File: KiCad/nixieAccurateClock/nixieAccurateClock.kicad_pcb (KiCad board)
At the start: 2 copper layers, 153 x 101.5 mm, 23 parts, among them J1 Conn_01x02_Pin, J2 Conn_01x02_Pin, J3 Conn_01x02_Pin, J4 Conn_Coaxial, Q1 PZTA42, SW1 SW_DIP_x02, U2 PX1125T

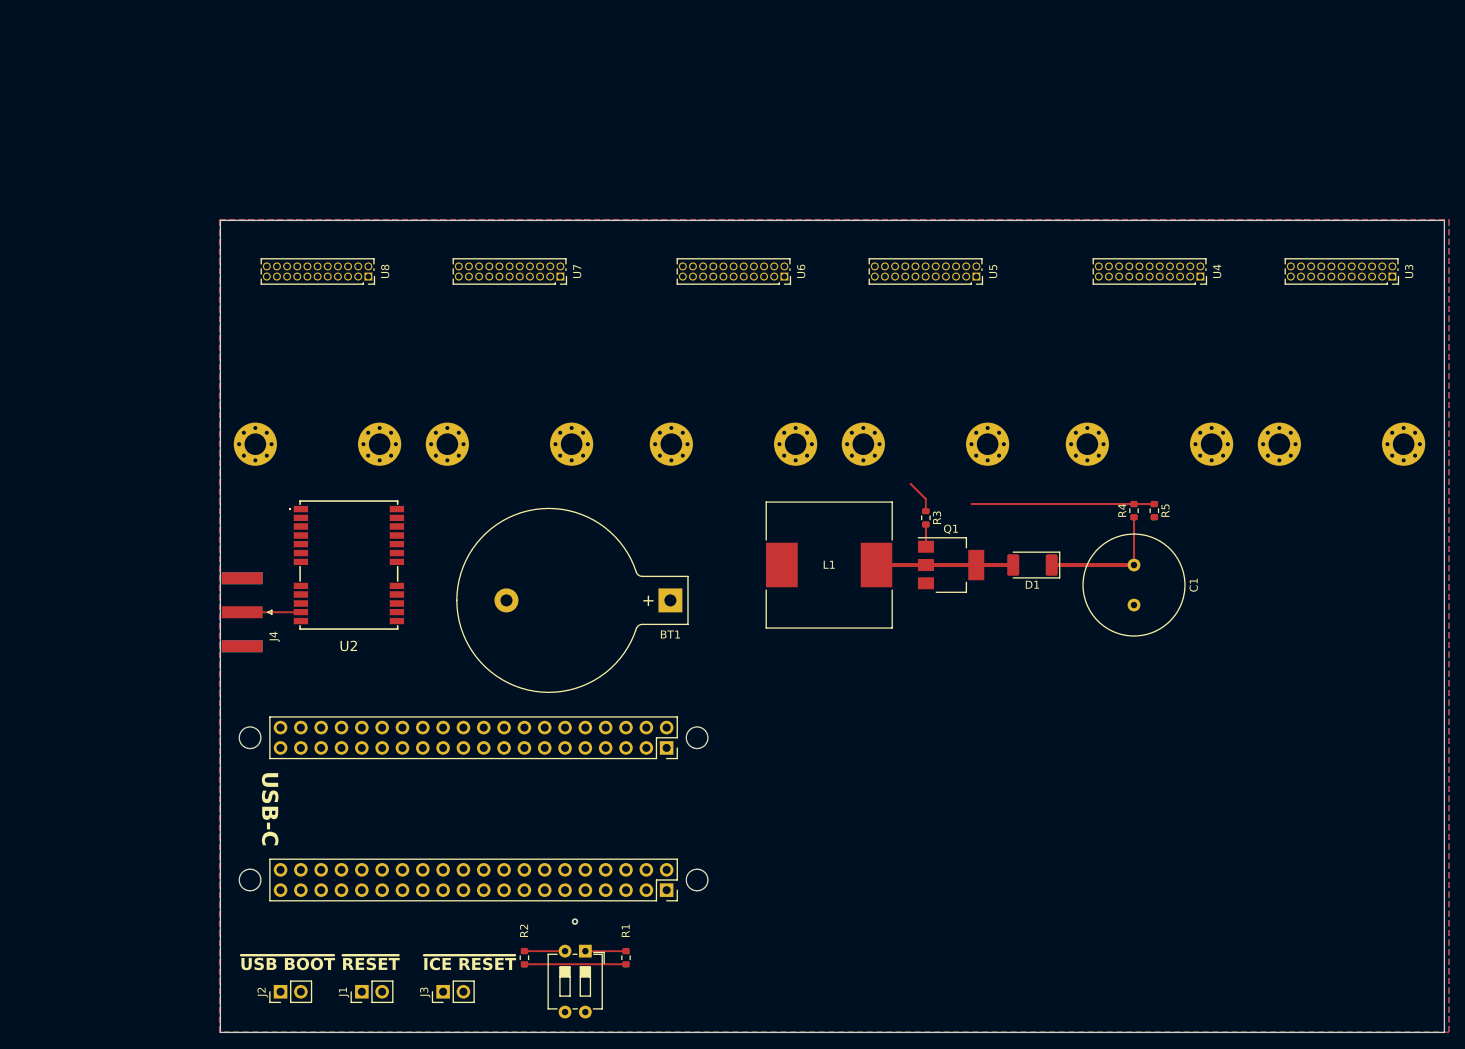
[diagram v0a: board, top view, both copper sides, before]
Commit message: WIP final feature push
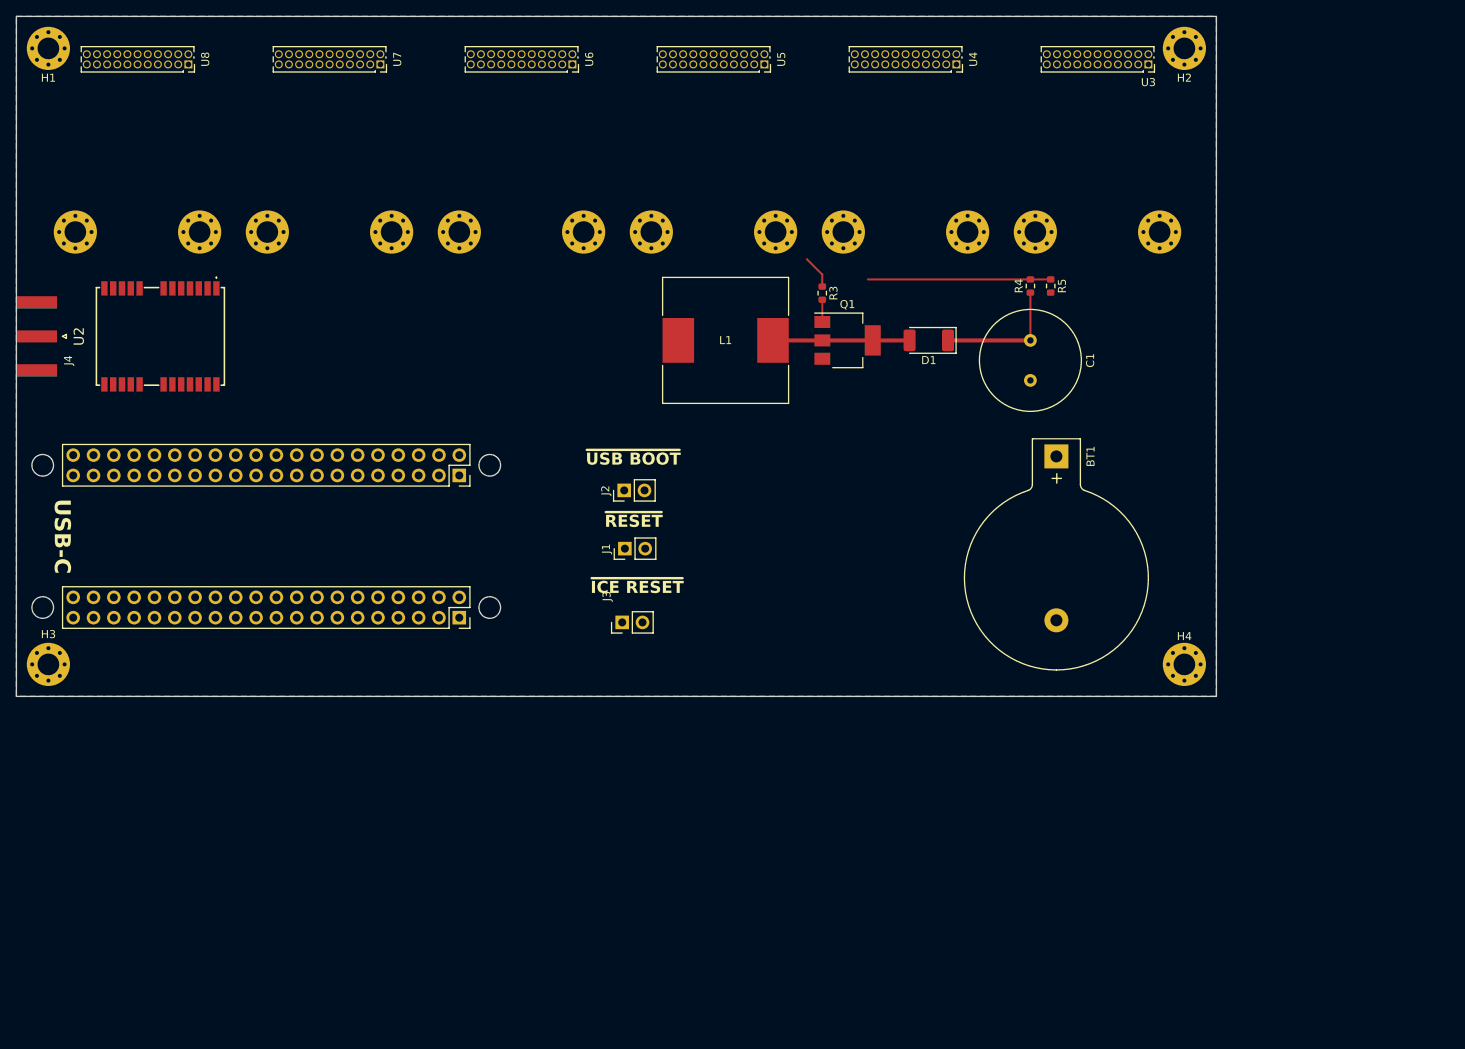
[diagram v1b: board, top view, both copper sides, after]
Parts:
- removed R1, R2: 100k, Resistor_SMD:R_0603_1608Metric
- removed SW1: SW_DIP_x02, Button_Switch_THT:SW_DIP_SPSTx02_Slide_6.7x6.64mm_W7.62mm_P2.54mm_LowProfile
- added H1: MountingHole_Pad, MountingHole:MountingHole_2.7mm_M2.5_Pad_Via, F.Cu at (4.00, 4.00)
- added H2: MountingHole_Pad, MountingHole:MountingHole_2.7mm_M2.5_Pad_Via, F.Cu at (146.0, 4.00)
- added H3: MountingHole_Pad, MountingHole:MountingHole_2.7mm_M2.5_Pad_Via, F.Cu at (4.00, 81.0)
- added H4: MountingHole_Pad, MountingHole:MountingHole_2.7mm_M2.5_Pad_Via, F.Cu at (146.0, 81.0)
- moved J2 76.0 mm to (76.0, 59.2)
- moved J1 64.4 mm to (76.1, 66.5)
- moved BT1 51.5 mm to (130.0, 55.0), turned to -90 degrees
- moved J3 51.3 mm to (75.7, 75.8)
- moved J4 43.0 mm to (2.54, 40.0)
- moved U1 42.8 mm to (32.5, 65.0)
- moved U3 40.4 mm to (141.5, 6.00)
- moved U4 40.4 mm to (117.5, 6.00)
- moved U5 37.5 mm to (93.5, 6.00)
- moved U6 37.5 mm to (69.5, 6.00)
- moved U2 37.0 mm to (18.0, 40.0), turned to 90 degrees
- moved U7 34.8 mm to (45.5, 6.00)
- moved U8 34.8 mm to (21.5, 6.00)
- moved R5 30.9 mm to (129.3, 33.7)
- moved C1 30.9 mm to (126.8, 40.5)
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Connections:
- net Net-(D1-A) renamed /High voltage supply/HV_BOOST
- U8 pad 10: unconnected-(U8-N_1-Pad10) -> /Nixies/N_1
- U8 pad 11: unconnected-(U8-N_6-Pad11) -> /Nixies/N_6
- U8 pad 13: unconnected-(U8-N_7-Pad13) -> /Nixies/N_7
- U8 pad 15: unconnected-(U8-N_8-Pad15) -> /Nixies/N_8
- U8 pad 17: unconnected-(U8-N_9-Pad17) -> /Nixies/N_9
- U8 pad 19: unconnected-(U8-N_0-Pad19) -> /Nixies/N_0
- U8 pad 3: unconnected-(U8-N_2-Pad3) -> /Nixies/N_2
- U8 pad 5: unconnected-(U8-N_3-Pad5) -> /Nixies/N_3
- U8 pad 7: unconnected-(U8-N_4-Pad7) -> /Nixies/N_4
- U8 pad 9: unconnected-(U8-N_5-Pad9) -> /Nixies/N_5
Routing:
- net +3.3V: track 12.7 -> 0.00 mm
- net Net-(J4-In): track 7.34 -> 0.00 mm
- net /DST_check: track 5.08 -> 0.00 mm
- net /DST_force: track 5.08 -> 0.00 mm
- net GND: vias 1 -> 0
- added copper zone on In1.Cu, net GND
- added copper zone on In2.Cu, net GND
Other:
- board size 153 x 101.5 mm -> 150 x 85 mm
- copper layers 2 -> 4
